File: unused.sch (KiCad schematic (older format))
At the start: 0 parts

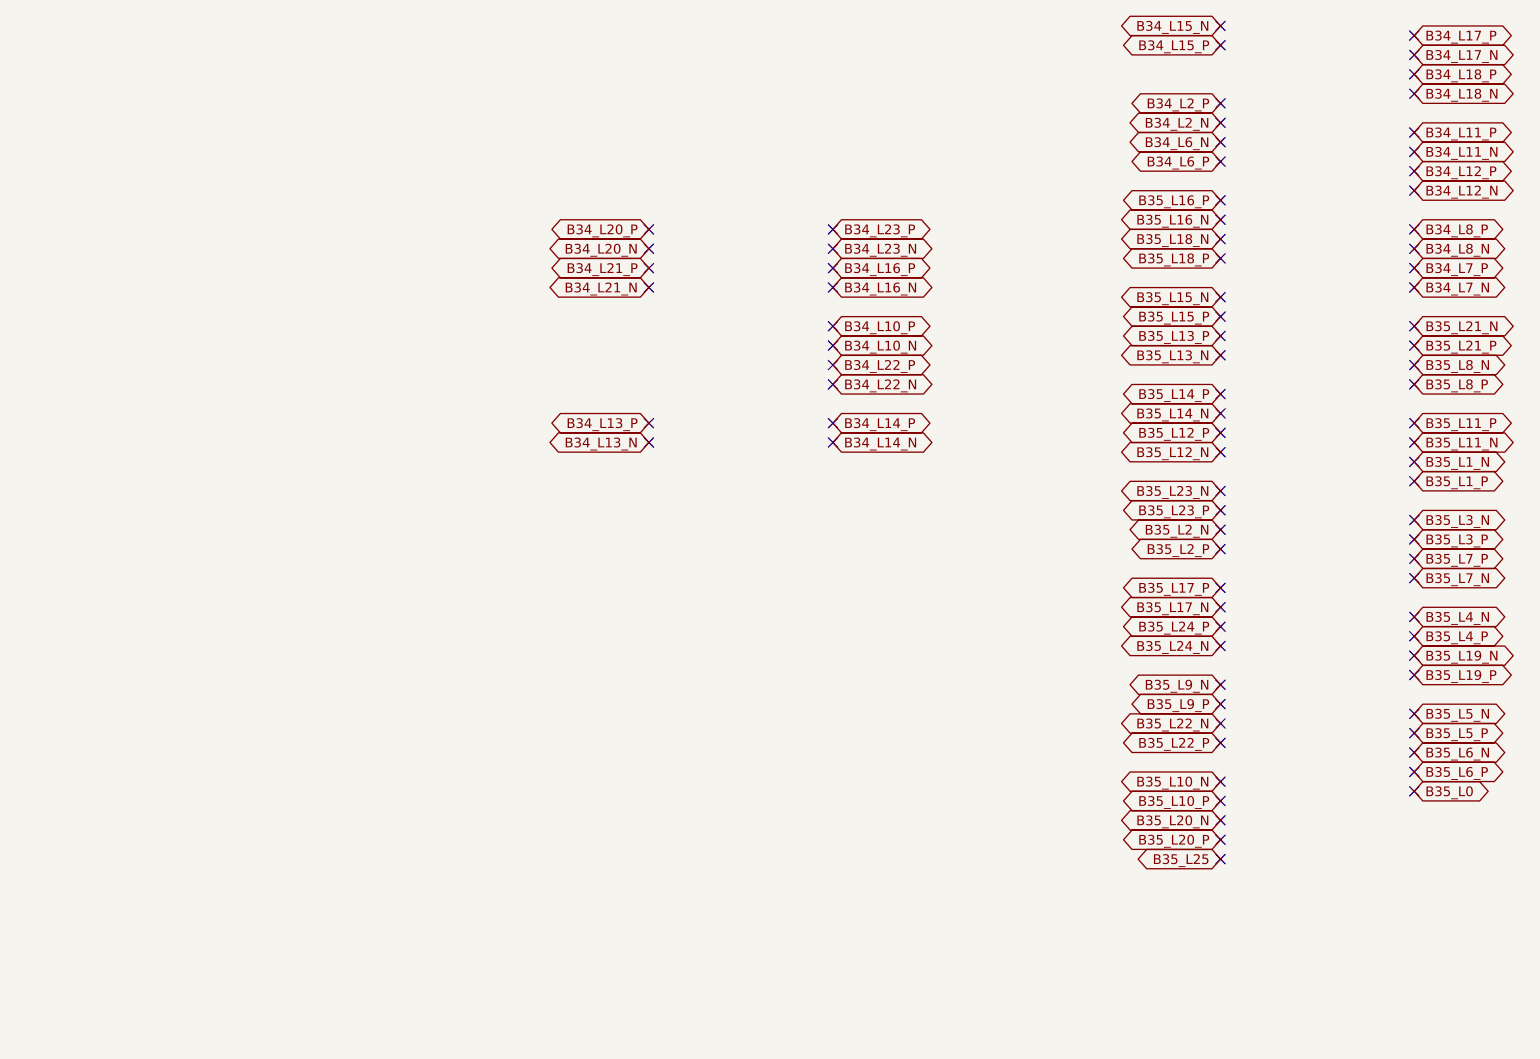
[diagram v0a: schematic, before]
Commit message: cont. work; all connections done now
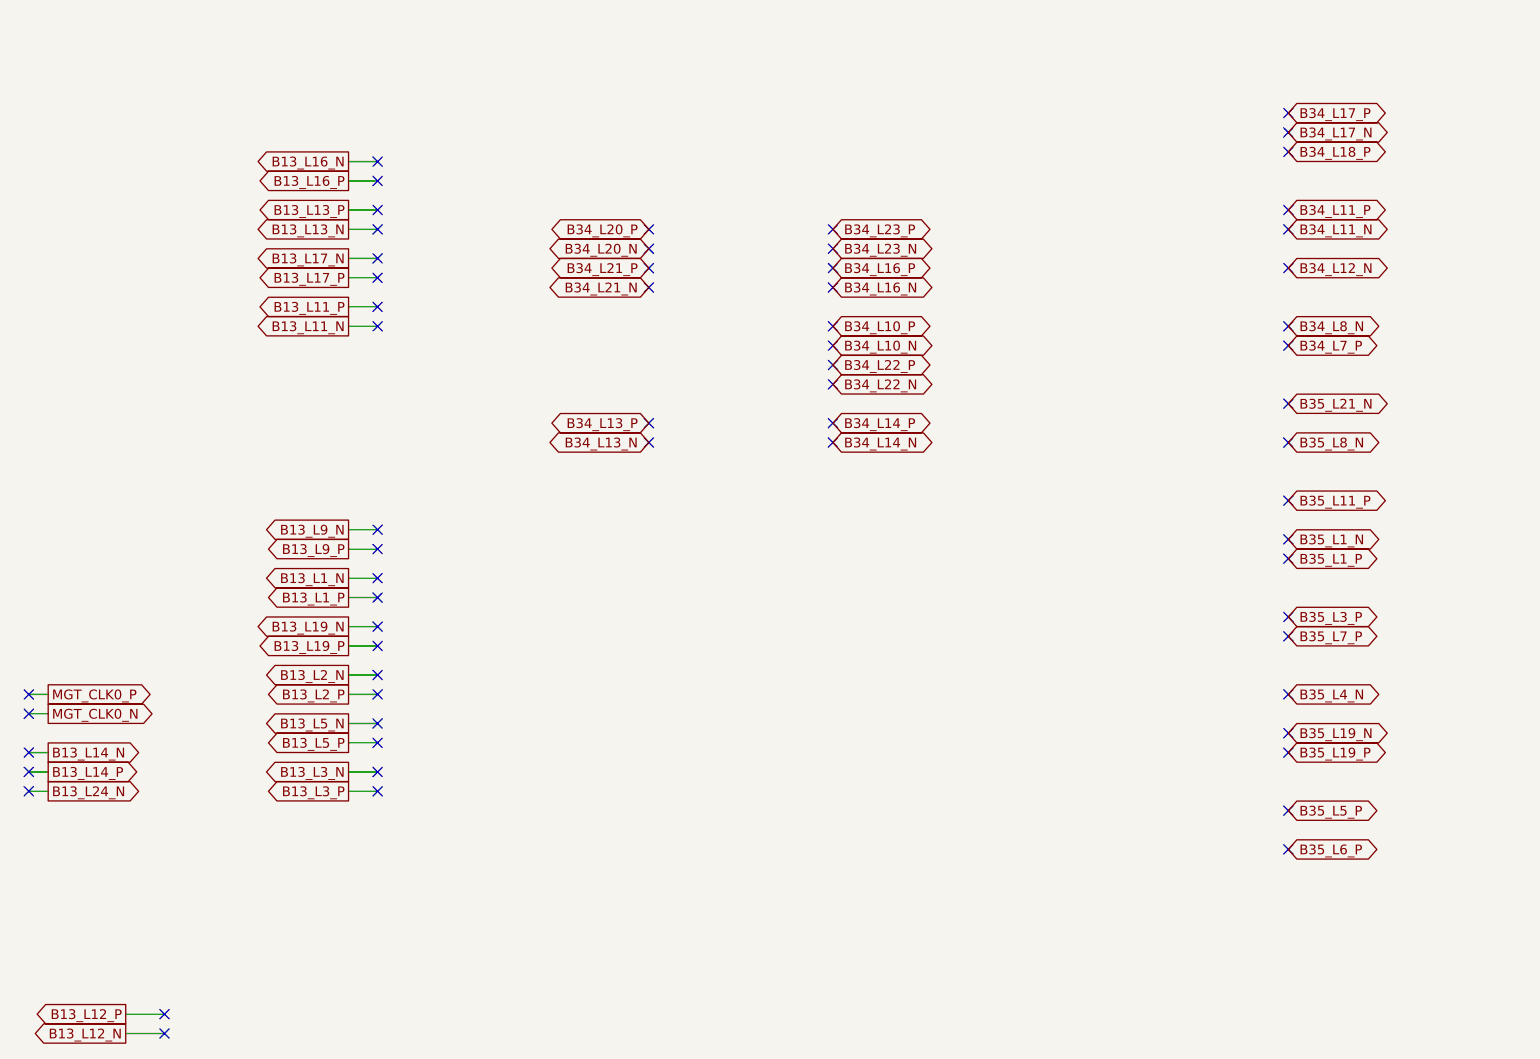
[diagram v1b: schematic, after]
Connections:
- no-connect marks 84 -> 63
